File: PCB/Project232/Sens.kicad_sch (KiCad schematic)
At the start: 19 parts, among them Q1 IRF3205, Q2 IRF3205, U3 ACS712, U4 ACS712, U6 IR2104

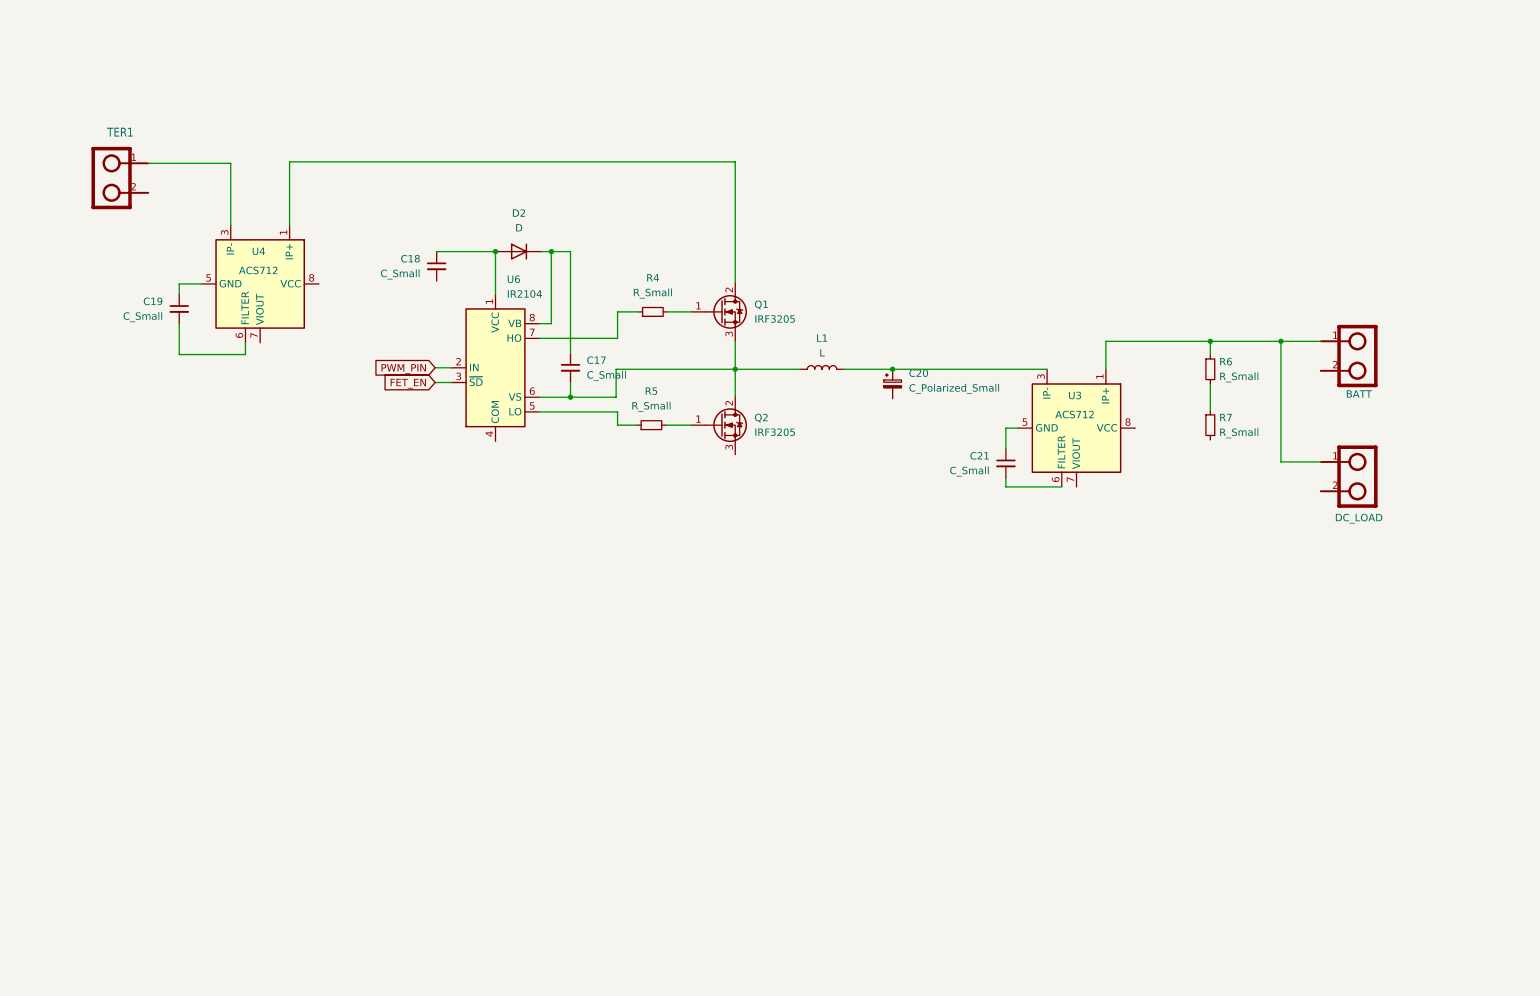
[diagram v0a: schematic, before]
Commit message: update test board and docs
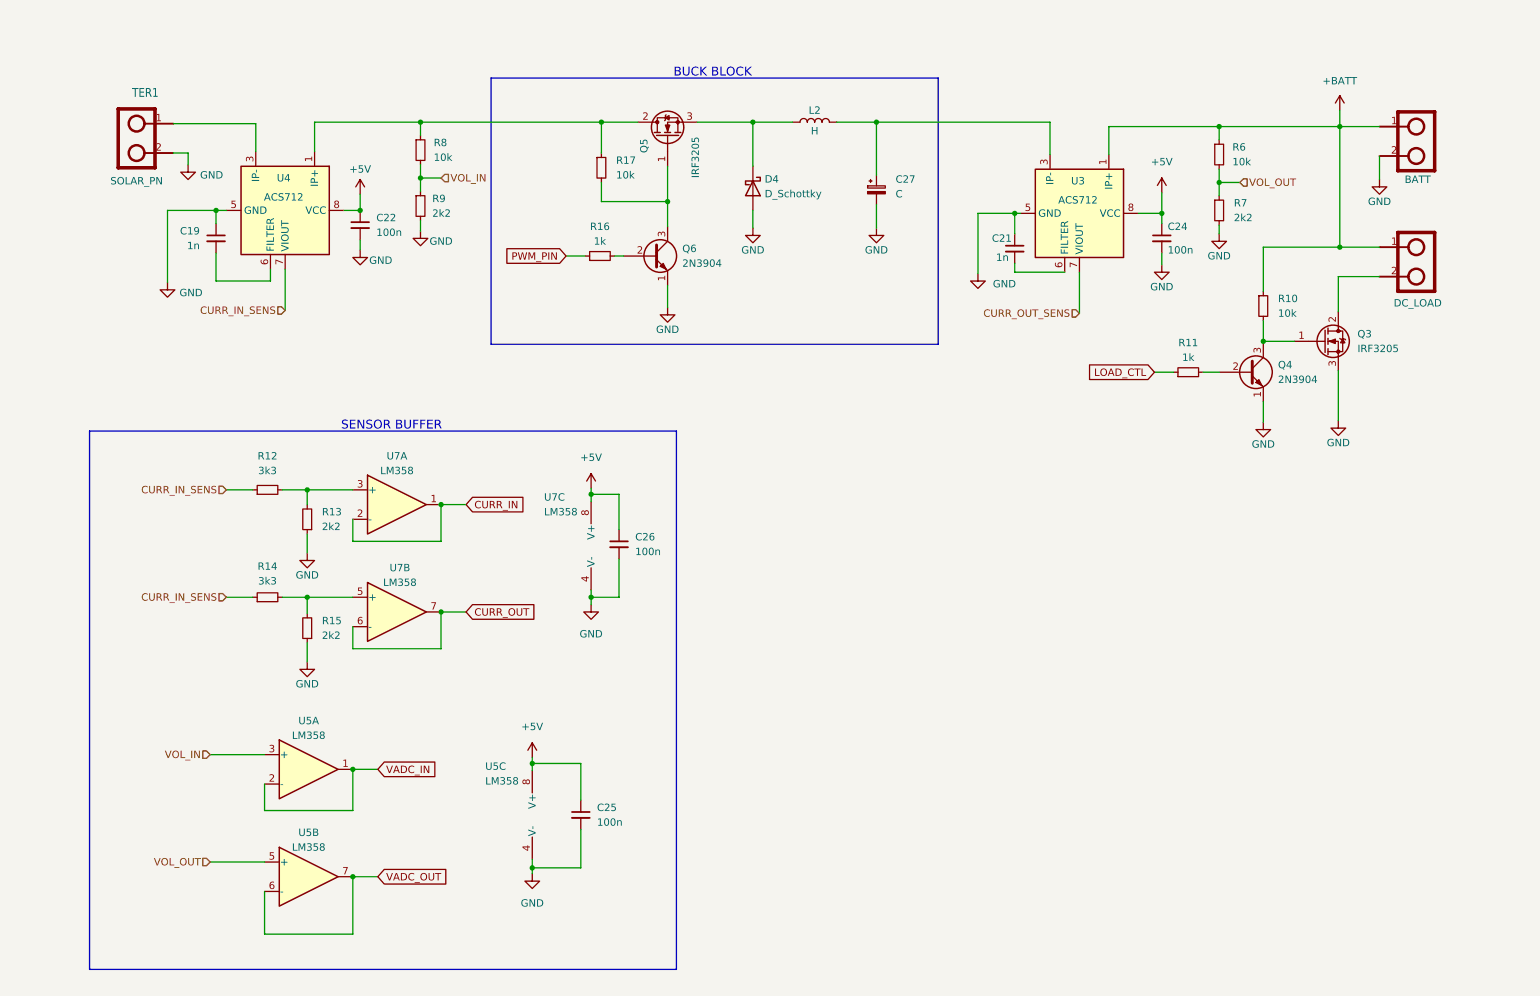
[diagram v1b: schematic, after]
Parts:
- removed C17, C18: C_Small, symbol Device:C_Small
- removed C20: C_Polarized_Small, symbol Device:C_Polarized_Small
- removed D2: D, symbol Device:D
- removed L1: L, symbol Device:L
- removed Q1, Q2: IRF3205, Package_TO_SOT_THT:TO-220-3_Vertical, symbol Transistor_FET:IRF3205
- removed R4, R5: R_Small, symbol Device:R_Small
- removed U6: IR2104, symbol Driver_FET:IR2104
- added C22, C24, C25, C26: 100n, symbol Device:C_Small
- added C27: C, symbol Device:C_Polarized_Small
- added D4: D_Schottky, symbol Device:D_Schottky
- added L2: H, symbol Device:L
- added Q3, Q5: IRF3205, Package_TO_SOT_THT:TO-220-3_Vertical, symbol Transistor_FET:IRF3205
- added Q4, Q6: 2N3904, Package_TO_SOT_THT:TO-92_Inline, symbol Transistor_BJT:2N3904
- added R10, R17, R8: 10k, symbol Device:R_Small
- added R11, R16: 1k, symbol Device:R_Small
- added R12, R14: 3k3, symbol Device:R_Small
- added R13, R15, R9: 2k2, symbol Device:R_Small
- added U5, U7: LM358, symbol Amplifier_Operational:LM358
- C19, C21: value C_Small -> 1n
- R6: value R_Small -> 10k
- R7: value R_Small -> 2k2
- TER1: value ~ -> SOLAR_PN
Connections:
- net PWM_PIN: now also R16.1
- net VOL_OUT: now reaches R6.2, R7.1
- net VOL_OUT: now also U5.5 (+)
- net GND: now reaches R7.2
- net GND: now also C19.1, C21.1, TER1.2, TER2.2, U3.5 (GND), U4.5 (GND), C22.2, C24.2, C25.2, C26.2, C27.2, D4.2 (A), Q3.3 (S), Q4.1 (E), Q6.1 (E), R13.1, R15.1, R9.2, U5.4 (V-), U7.4 (V-)
- net at U3.3 (IP-), U3.4 (IP-): now also C27.1, L2.2
- net at U4.1 (IP+), U4.2 (IP+): now also Q5.2 (D), R17.1, R8.1
- net +BATT: now reaches R6.1, TER2.1, TER3.1, U3.1 (IP+), U3.2 (IP+)
- net +BATT: now also R10.1
- net at TER3.2: now also Q3.2 (D)
- net CURR_OUT_SENS: now reaches U3.7 (VIOUT)
- net +5V: now reaches U3.8 (VCC)
- net +5V: now also U4.8 (VCC), C22.1, C24.1, C25.1, C26.1, U5.8 (V+), U7.8 (V+)
- net CURR_IN_SENS: now reaches U4.7 (VIOUT)
- net CURR_IN_SENS: now also R12.1, R14.1
- new net: Q5.1 (G), Q6.3 (C), R17.2
- new net: R12.2, R13.2, U7.3 (+)
- new net: Q4.2 (B), R11.2
- new net: Q3.1 (G), Q4.3 (C), R10.2
- new net: R14.2, R15.2, U7.5 (+)
- new net: D4.1 (K), L2.1, Q5.3 (S)
- new net: Q6.2 (B), R16.2
- new net CURR_IN: U7.1, U7.2 (-)
- new net CURR_OUT: U7.6 (-), U7.7
- new net LOAD_CTL: R11.1
- new net VADC_IN: U5.1, U5.2 (-)
- new net VADC_OUT: U5.6 (-), U5.7
- new net VOL_IN: R8.2, R9.1, U5.3 (+)
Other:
- note added: "BUCK BLOCK"
- note added: "SENSOR BUFFER"
- moved on the sheet: C19, C21, R6, R7, TER1, U3, U4

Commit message: Update PCB
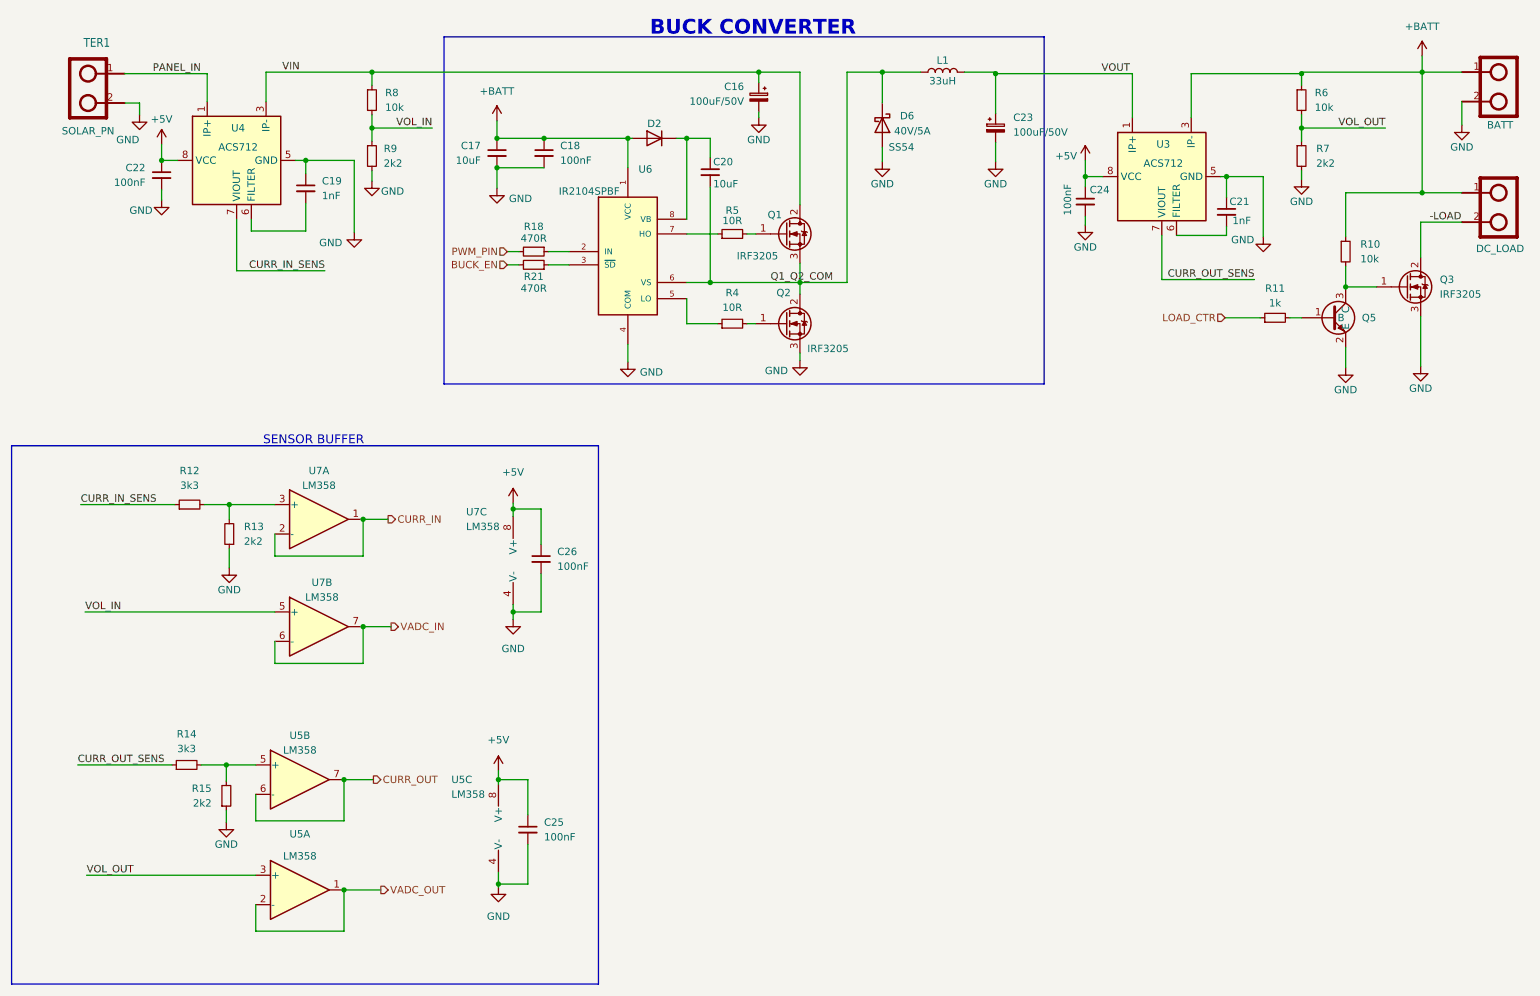
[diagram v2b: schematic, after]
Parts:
- removed C27: C, symbol Device:C_Polarized_Small
- removed D4: D_Schottky, symbol Device:D_Schottky
- removed L2: H, symbol Device:L
- removed Q4, Q6: 2N3904, Package_TO_SOT_THT:TO-92_Inline, symbol Transistor_BJT:2N3904
- removed Q5: IRF3205, Package_TO_SOT_THT:TO-220-3_Vertical, symbol Transistor_FET:IRF3205
- removed R16: 1k, symbol Device:R_Small
- removed R17: 10k, symbol Device:R_Small
- added C16, C23: 100uF/50V, Capacitor_SMD:CP_Elec_8x10.5, symbol Device:C_Polarized_Small
- added C17, C20: 10uF, Capacitor_SMD:C_0402_1005Metric, symbol Device:C_Small
- added C18: 100nF, Capacitor_SMD:C_0402_1005Metric, symbol Device:C_Small
- added D2: 1N5819W, Diode_SMD:D_SOD-123, symbol Device:D
- added D6: 40V/5A, Diode_SMD:D_SMC, symbol Diode:B350
- added L1: 33uH, Induc_THT:Inductor_33uH_5A_THT, symbol Device:L
- added Q1, Q2: IRF3205, Package_TO_SOT_THT:TO-220-3_Vertical, symbol Transistor_FET:IRF3205
- added Q5: ~, Package_TO_SOT_SMD:SOT-23, symbol NPN_Trans_2SC1815:2SC1815
- added R18, R21: 470R, Resistor_SMD:R_0603_1608Metric, symbol Device:R_Small
- added R4, R5: 10R, Resistor_SMD:R_0603_1608Metric, symbol Device:R_Small
- added U6: IR2104SPBF, IR2104SPBF:SOIC127P600X175-8N, symbol IR2104SPBF:IR2104SPBF
- C19, C21: value 1n -> 1nF; footprint (none) -> Capacitor_SMD:C_0402_1005Metric
- C22, C24, C25, C26: value 100n -> 100nF; footprint (none) -> Capacitor_SMD:C_0402_1005Metric
- R10, R11, R12, R13, R14, R15, R6, R7, R8, R9: footprint (none) -> Resistor_SMD:R_0603_1608Metric
- TER1, TER2, TER3: footprint Project232:DOMI-2 -> TerminalBlock:TerminalBlock_bornier-2_P5.08mm
- U5, U7: footprint (none) -> Package_SO:SOIC-8_3.9x4.9mm_P1.27mm
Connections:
- net +BATT: now also U3.3 (IP-), U3.4 (IP-), C17.1, C18.1, D2.2 (A), U6.1 (VCC); no longer U3.1 (IP+), U3.2 (IP+)
- net CURR_IN_SENS: no longer R14.1
- net CURR_OUT: now also U5.6 (-), U5.7; no longer U7.6 (-), U7.7
- net CURR_OUT_SENS: now also R14.1
- net GND: now also C16.2, C17.2, C18.2, C23.2, D6.2 (A), Q2.3 (S), Q5.2 (E), U6.4 (COM)
- net PWM_PIN: now also R18.2
- net VADC_IN: now also U7.6 (-), U7.7; no longer U5.1, U5.2 (-)
- net VADC_OUT: now also U5.1, U5.2 (-); no longer U5.6 (-), U5.7
- net VOL_IN: now also U7.5 (+); no longer U5.3 (+)
- net VOL_OUT: now also U5.3 (+); no longer U5.5 (+)
- net PANEL_IN: now reaches U4.1 (IP+), U4.2 (IP+)
- net PANEL_IN: now also TER1.1; no longer R8.1
- net at R11.2: now also Q5.1 (B)
- net at Q3.1 (G), R10.2: now also Q5.3 (C)
- net VIN: now reaches U4.3 (IP-), U4.4 (IP-)
- net VIN: now also R8.1, C16.1, Q1.2 (D); no longer TER1.1
- net -LOAD: now reaches Q3.2 (D), TER3.2
- net at R14.2, R15.2: now also U5.5 (+); no longer U7.5 (+)
- net LOAD_CTL renamed LOAD_CTR
- new net: C20.1, D2.1 (K), U6.8 (VB)
- new net: R18.1, U6.2 (IN)
- new net: Q2.1 (G), R4.2
- new net: R5.1, U6.7 (HO)
- new net: Q1.1 (G), R5.2
- new net: R4.1, U6.5 (LO)
- new net: R21.1, U6.3 (~{SD})
- new net BUCK_EN: R21.2
- new net Q1_Q2_COM: C20.2, D6.1 (K), L1.1, Q1.3 (S), Q2.2 (D), U6.6 (VS)
- new net VOUT: C23.1, L1.2, U3.1 (IP+), U3.2 (IP+)
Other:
- note added: "BUCK CONVERTER"
- note removed: "BUCK BLOCK"
- moved on the sheet: C19, C21, C22, C24, C25, C26, Q3, R10, R11, R12, R13, R14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
